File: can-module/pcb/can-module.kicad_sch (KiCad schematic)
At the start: 52 parts, among them J1 Conn_01x04_Socket, J2 Conn_01x08_Socket, J3 Conn_01x02_Socket, U1 NID5100GWH, U2 MIC5365-3.3YC5, U3 ATA6560-GBQW-N, U4 PIC32CM1216JH01048-I_U5B

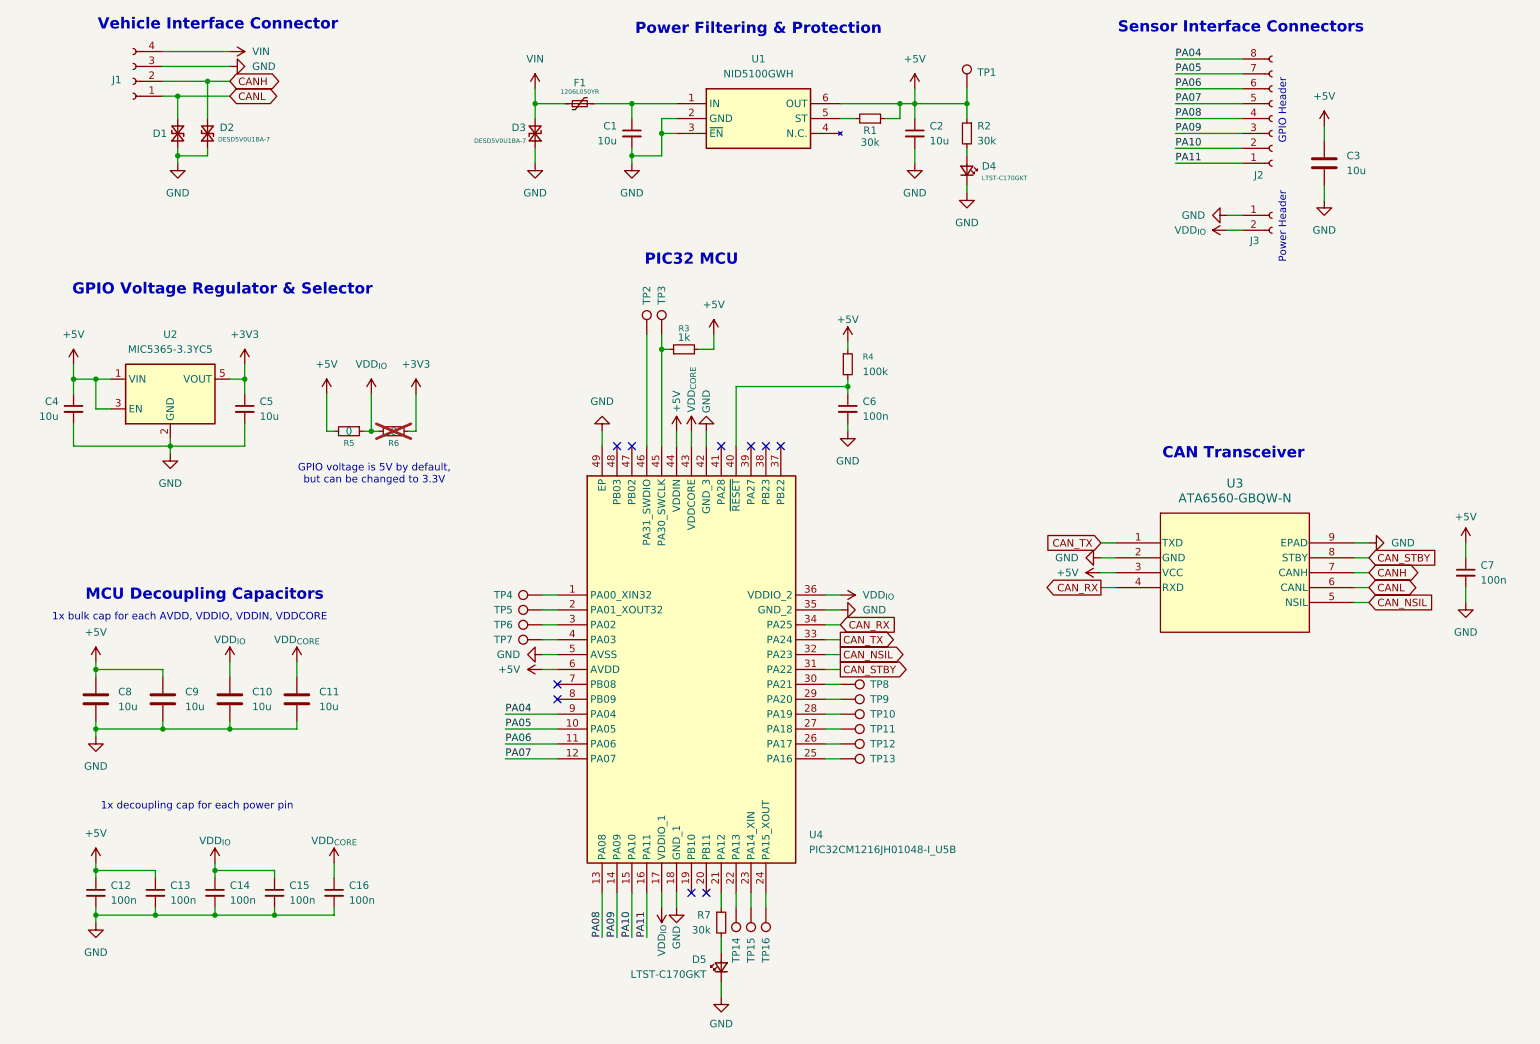
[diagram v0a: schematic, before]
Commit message: can-module: Change programming header to be through hole for easier access
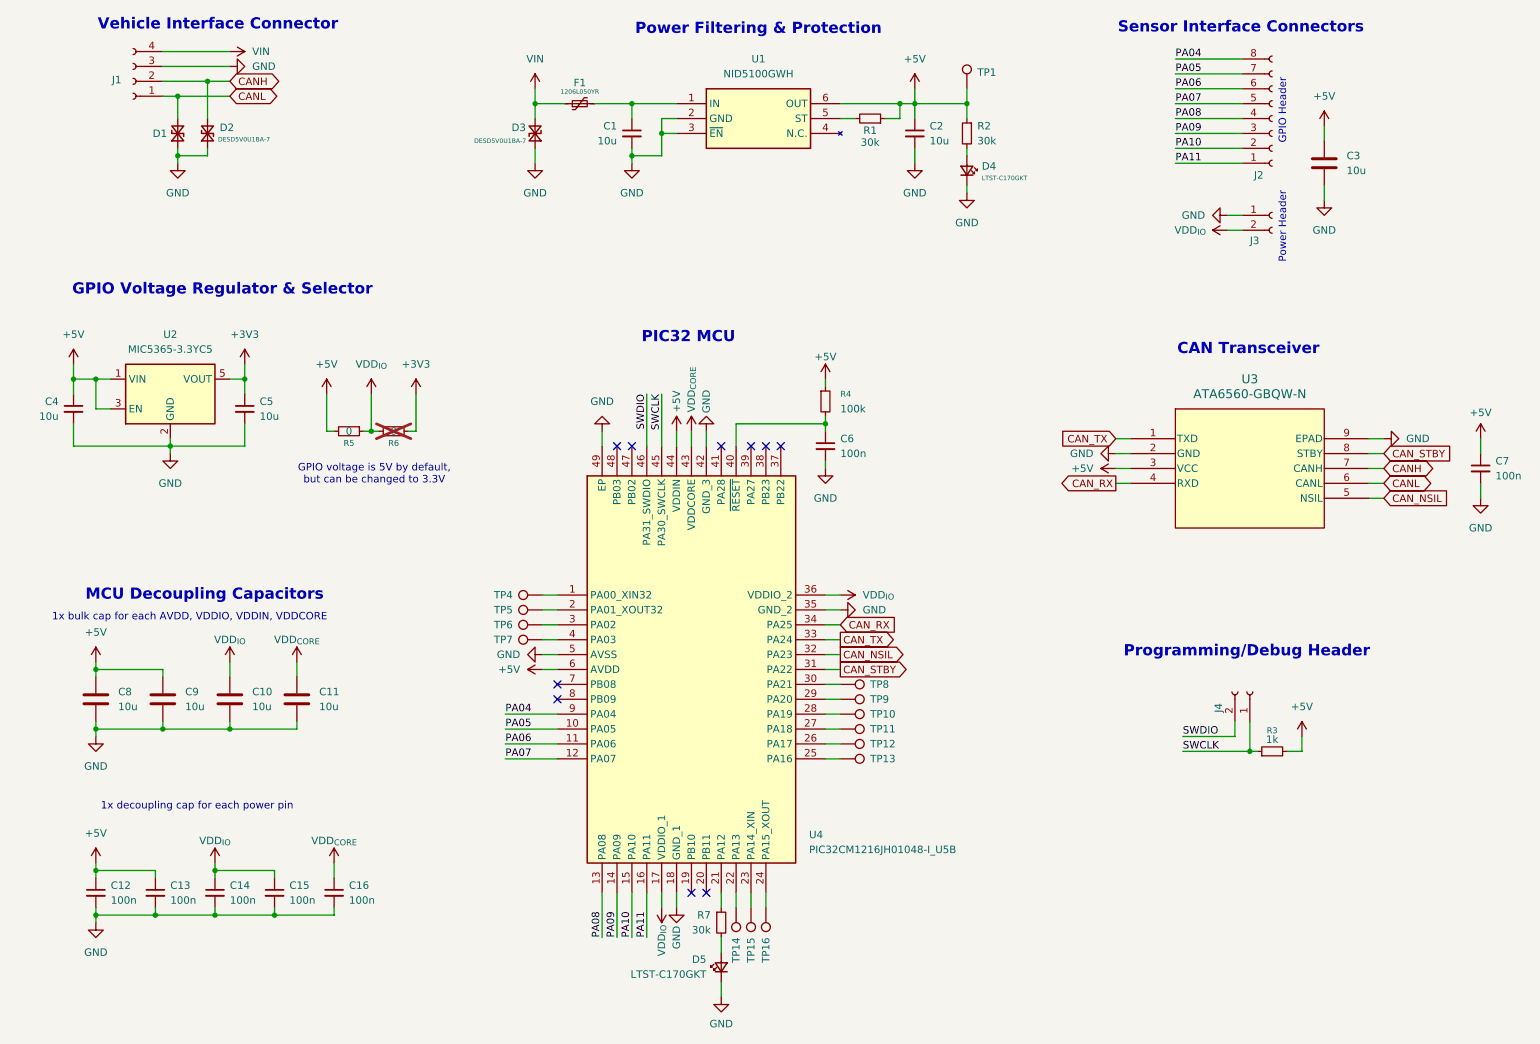
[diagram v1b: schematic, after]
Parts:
- removed TP2, TP3: TestPoint, TestPoints:TestPoint_Pad_D1.0mm_TightSpacing, symbol Connector:TestPoint
- added J4: Conn_01x02_Socket, Connector_PinHeader_1.27mm:PinHeader_1x02_P1.27mm_Vertical, symbol Connector:Conn_01x02_Socket
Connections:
- net SWCLK: now reaches R3.1, U4.45 (PA30_SWCLK)
- net SWCLK: now also J4.1 (Pin_1)
- net SWDIO: now reaches U4.46 (PA31_SWDIO)
- net SWDIO: now also J4.2 (Pin_2)
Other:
- note added: "Programming/Debug Header"
- moved on the sheet: C6, C7, R3, R4, U3

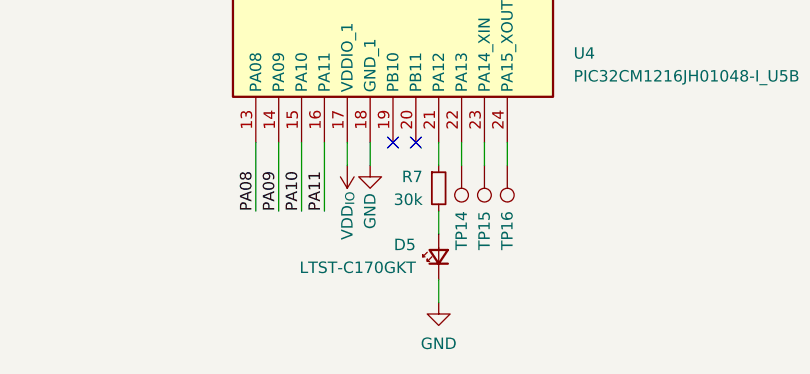
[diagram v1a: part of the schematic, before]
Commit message: can-module: Flip indicator LED around so that anode is always 5V
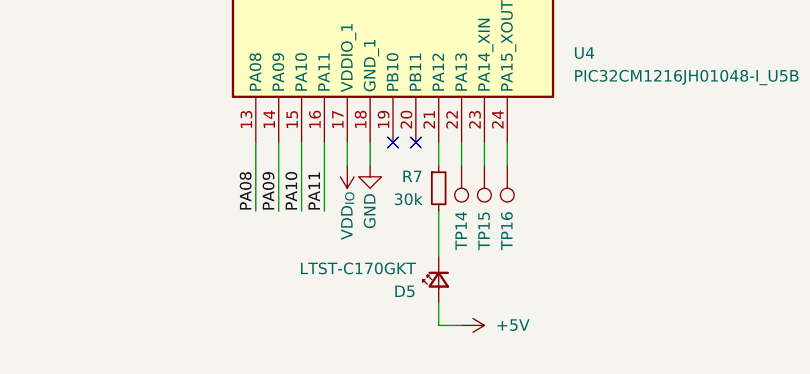
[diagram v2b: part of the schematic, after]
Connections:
- net +5V: now also D5.2 (A)
- net GND: no longer D5.1 (K)
- net at R7.2: now also D5.1 (K); no longer D5.2 (A)
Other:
- moved on the sheet: D5
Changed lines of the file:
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@@
 	(wire
 		(pts
-			(xy 142.24 176.53) (xy 142.24 179.07)
+			(xy 142.24 176.53) (xy 142.24 181.61)
 		)
 		(stroke
@@
 	(wire
 		(pts
+			(xy 144.78 189.23) (xy 142.24 189.23)
+		)
+		(stroke
+			(width 0)
+			(type default)
+		)
+	)
+	(wire
+		(pts
 			(xy 252.73 99.06) (xy 255.27 99.06)
 		)
@@
 	(wire
 		(pts
-			(xy 142.24 184.15) (xy 142.24 186.69)
+			(xy 132.08 36.83) (xy 134.62 36.83)
 		)
 		(stroke
@@
 	(wire
 		(pts
-			(xy 132.08 36.83) (xy 134.62 36.83)
+			(xy 46.99 130.81) (xy 46.99 132.08)
 		)
 		(stroke
@@
 	(wire
 		(pts
-			(xy 46.99 130.81) (xy 46.99 132.08)
+			(xy 46.99 25.4) (xy 58.42 25.4)
 		)
 		(stroke
@@
 	(wire
 		(pts
-			(xy 46.99 25.4) (xy 58.42 25.4)
+			(xy 142.24 189.23) (xy 142.24 186.69)
 		)
 		(stroke
@@
 	(symbol
 		(lib_id "Device:LED_Small")
-		(at 142.24 181.61 90)
+		(at 142.24 184.15 90)
+		(mirror x)
 		(unit 1)
 		(exclude_from_sim no)
@@
 		(dnp no)
 		(property "Reference" "D5"
-			(at 139.7 180.2764 90)
+			(at 139.7 185.4836 90)
 			(effects
 				(font
@@
 		)
 		(property "Value" "LTST-C170GKT"
-			(at 139.7 182.8164 90)
+			(at 139.7 182.9436 90)
 			(effects
 				(font
@@
 		)
 		(property "Footprint" "LED_SMD:LED_0805_2012Metric"
-			(at 142.24 181.61 90)
+			(at 142.24 184.15 90)
 			(effects
 				(font
@@
 		)
 		(property "Datasheet" "~"
-			(at 142.24 181.61 90)
+			(at 142.24 184.15 90)
 			(effects
 				(font
@@
 		)
 		(property "Description" "Light emitting diode, small symbol"
-			(at 142.24 181.61 0)
+			(at 142.24 184.15 0)
 			(effects
 				(font
@@
 		)
 		(property "Sim.Pin" "1=K 2=A"
-			(at 142.24 181.61 0)
+			(at 142.24 184.15 0)
 			(effects
 				(font
@@
 		)
 		(instances
-			(project ""
+			(project "can-module"
 				(path "/40cb4209-4f7f-4a38-b0f0-dee54a92ee91"
 					(reference "D5")
@@
 	)
 	(symbol
-		(lib_id "power:GND")
-		(at 142.24 186.69 0)
-		(mirror y)
-		(unit 1)
-		(exclude_from_sim no)
-		(in_bom yes)
-		(on_board yes)
-		(dnp no)
-		(property "Reference" "#PWR046"
-			(at 142.24 193.04 0)
-			(effects
-				(font
-					(size 1.27 1.27)
-				)
-				(hide yes)
-			)
-		)
-		(property "Value" "GND"
-			(at 142.24 191.262 0)
-			(effects
-				(font
-					(size 1.27 1.27)
-				)
-			)
-		)
-		(property "Footprint" ""
-			(at 142.24 186.69 0)
-			(effects
-				(font
-					(size 1.27 1.27)
-				)
-				(hide yes)
-			)
-		)
-		(property "Datasheet" ""
-			(at 142.24 186.69 0)
-			(effects
-				(font
-					(size 1.27 1.27)
-				)
-				(hide yes)
-			)
-		)
-		(property "Description" "Power symbol creates a global label with name \"GND\" , ground"
-			(at 142.24 186.69 0)
-			(effects
-				(font
-					(size 1.27 1.27)
-				)
-				(hide yes)
-			)
-		)
-		(pin "1"
-		)
-		(instances
-			(project "can-module"
-				(path "/40cb4209-4f7f-4a38-b0f0-dee54a92ee91"
-					(reference "#PWR046")
-					(unit 1)
-				)
-			)
-		)
-	)
-	(symbol
 		(lib_id "Device:C")
 		(at 58.42 135.89 0)
@@
 					(unit 1)
 				)
+			)
+		)
+	)
+	(symbol
+		(lib_id "power:+5V")
+		(at 144.78 189.23 270)
+		(unit 1)
+		(exclude_from_sim no)
+		(in_bom yes)
+		(on_board yes)
+		(dnp no)
+		(fields_autoplaced yes)
+		(property "Reference" "#PWR013"
+			(at 140.97 189.23 0)
+			(effects
+				(font
+					(size 1.27 1.27)
+				)
+				(hide yes)
+			)
+		)
+		(property "Value" "+5V"
+			(at 148.59 189.2299 90)
+			(effects
+				(font
+					(size 1.27 1.27)
+				)
+				(justify left)
+			)
+		)
+		(property "Footprint" ""
+			(at 144.78 189.23 0)
+			(effects
+				(font
+					(size 1.27 1.27)
+				)
+				(hide yes)
+			)
+		)
+		(property "Datasheet" ""
+			(at 144.78 189.23 0)
+			(effects
+				(font
+					(size 1.27 1.27)
+				)
+				(hide yes)
+			)
+		)
+		(property "Description" "Power symbol creates a global label with name \"+5V\""
+			(at 144.78 189.23 0)
+			(effects
+				(font
+					(size 1.27 1.27)
+				)
+				(hide yes)
+			)
+		)
+		(pin "1"
+		)
+		(instances
+			(project "can-module"
+				(path "/40cb4209-4f7f-4a38-b0f0-dee54a92ee91"
+					(reference "#PWR013")
+					(unit 1)
+				)
